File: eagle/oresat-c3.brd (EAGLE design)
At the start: 99.8 x 94.6 mm, 419 parts, among them IC2 STM32F439VIT6_PORT_BREAKOUT, J5 ORESAT-DEBUG-CONNECTOR-ALL, J6 J-SAMTEC-TFM-120-X1-XXX-D-RA, Q1 MOSFET-PCH-SOT23-6, Q10 PMOS, Q11 FDMQ86530L, Q12 DMP2240UDM-7, Q13 DMP2240UDM-7, Q14 FDMQ86530L, Q2 NTR4101, Q4 P-CH, Q5 N-CH, Q6 DMP2240UDM-7, Q7 BFPXXXF, Q8 DMP2240UDM-7, Q9 BFPXXXF, U1 MAX892LEUA+T21-0036K-L, U10 SI4112, U11 U-ONSEMI-AX5043, U12 LP2985AIM5-1.8_NOPB, U13 U-ONSEMI-AX5043, U14 LP2985AIM5-1.8_NOPB, U15 Qorvo 856930, U16 MAC-24+, U17 BP0805A1308, U18 B8666, U19 BP0805A1308, U2 TCAN330, U20 BGB7XXL7ESD, U21 BP0805A1308, U22 TLV7041DCKRYC5, U23 LP2985AIM5-2.5_NOPB, U24 MAX941EUA+, U25 SN74LVC1G32QDBVRQ1, U26 TPS62112, U27 TPS259620, U28 LP2985AIM5-3.3_NOPB, U29 SN74LVC1G11IDCKRQ1, U3 TCAN330, U30 U-TQP7M9105, U31 BDCN-20-13+, U32 LT5534, U33 LT5534, U34 Micro Crystal RV-3028-C7, U35 FM24CL64B-DGTR, U4 TPS259621, U5 TPS62111RSA, U6 LP2985AIM5-2.5_NOPB, U7 TLV1704AMPWPSEP, U8 QPC1022, U9 SFEM016GB1EM1TO-A-HG-111-STD, X1 ECS-160-10-36Q-ES-TR_16MHZ, X2 ABS07-32.768KHZ-T-SMD-2, X3 TAITIEN-TY, X4 TAITIEN-TY

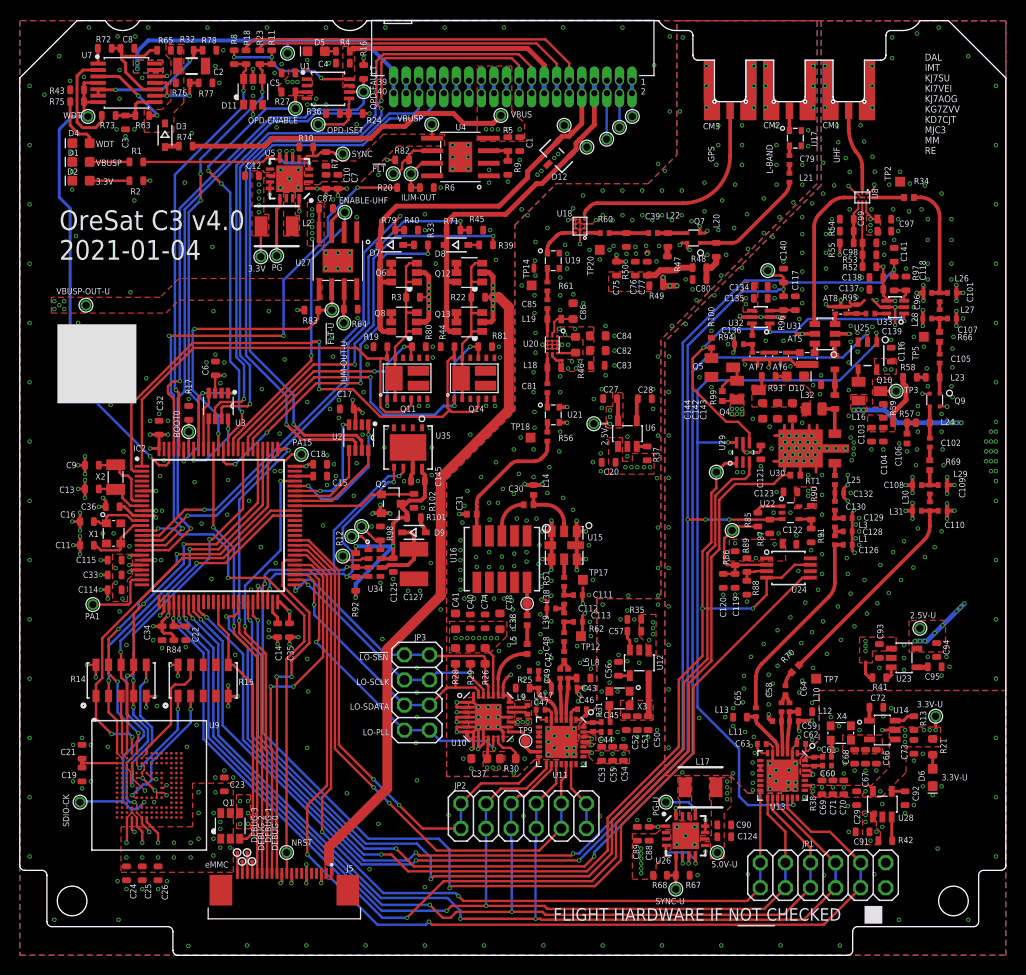
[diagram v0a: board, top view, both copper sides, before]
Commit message: Updated date BOM for C3 V4, fixed some parts for future V5.
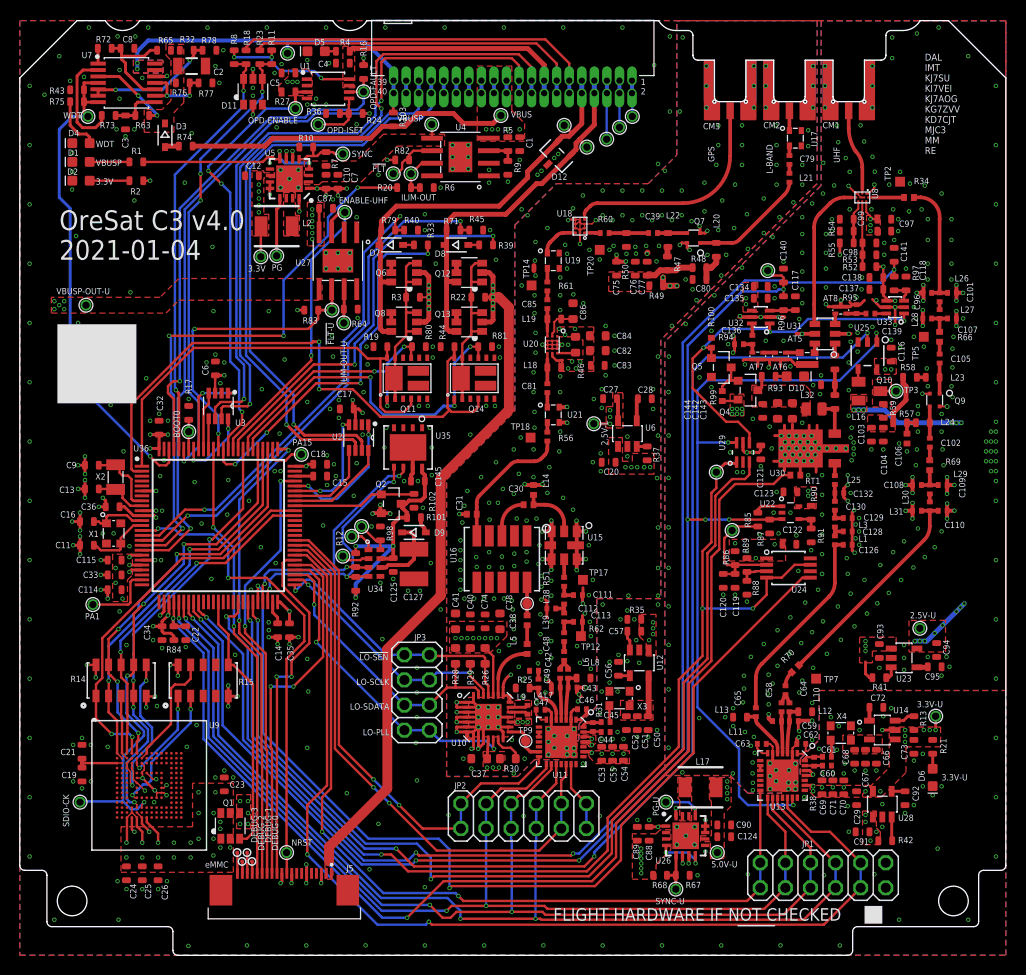
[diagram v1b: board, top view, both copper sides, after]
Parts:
- added R103: 100k, C3_SamacSys_Parts:.0603-C-NOSILK
- C144: device oresat-rcl:.0603-B-NOSILK -> oresat-rcl:.0603-C-NOSILK
- Q4: value P-CH -> NTR4101; device transistor-small-signal:SOT23 -> Q-MOSFET-PCH-SOT23-3:SOT23-3
- Q5: value N-CH -> PM45EN; device transistor-small-signal:SOT23 -> Q-MOSFET-NCH-SOT23-3:SOT23-3
- R101: value 100 -> 150
- R21: device oresat-rcl:.0603-B-NOSILK -> C3_SamacSys_Parts:.0603-C-NOSILK
- R52, R53, R54, R55, R93, R96, R97: device oresat-rcl:.0603-C-NOSILK -> C3_SamacSys_Parts:.0603-C-NOSILK
- R82: value NP/10K -> 10K
- R94, R95: value 47 -> 50
- U20: value BGB7XXL7ESD -> BGB741L7ESD
- moved Q5 0.10 mm to (71.0, 59.5)
- renumbered IC2 to U36
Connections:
- net !SD: now also R103.1
- net VBUS: now also R103.2
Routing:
- net !SD: track 33.1 -> 35.0 mm
